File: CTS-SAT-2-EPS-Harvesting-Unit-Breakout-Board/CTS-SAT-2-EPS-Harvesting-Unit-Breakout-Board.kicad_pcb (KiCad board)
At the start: 2 copper layers, 60.2 x 19 mm, 9 parts, among them J1 Conn_01x02_Pin, U1 MAX9922EUB+T

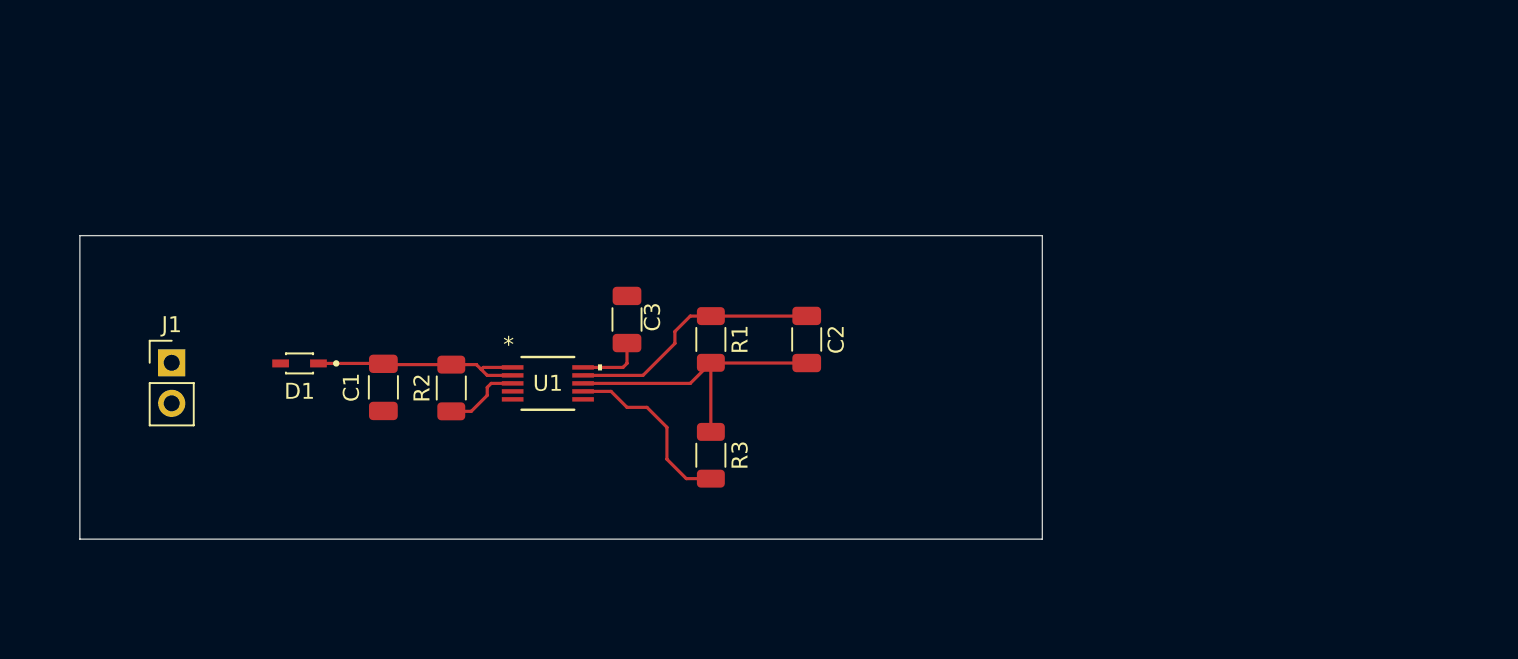
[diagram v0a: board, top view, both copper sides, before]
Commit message: update
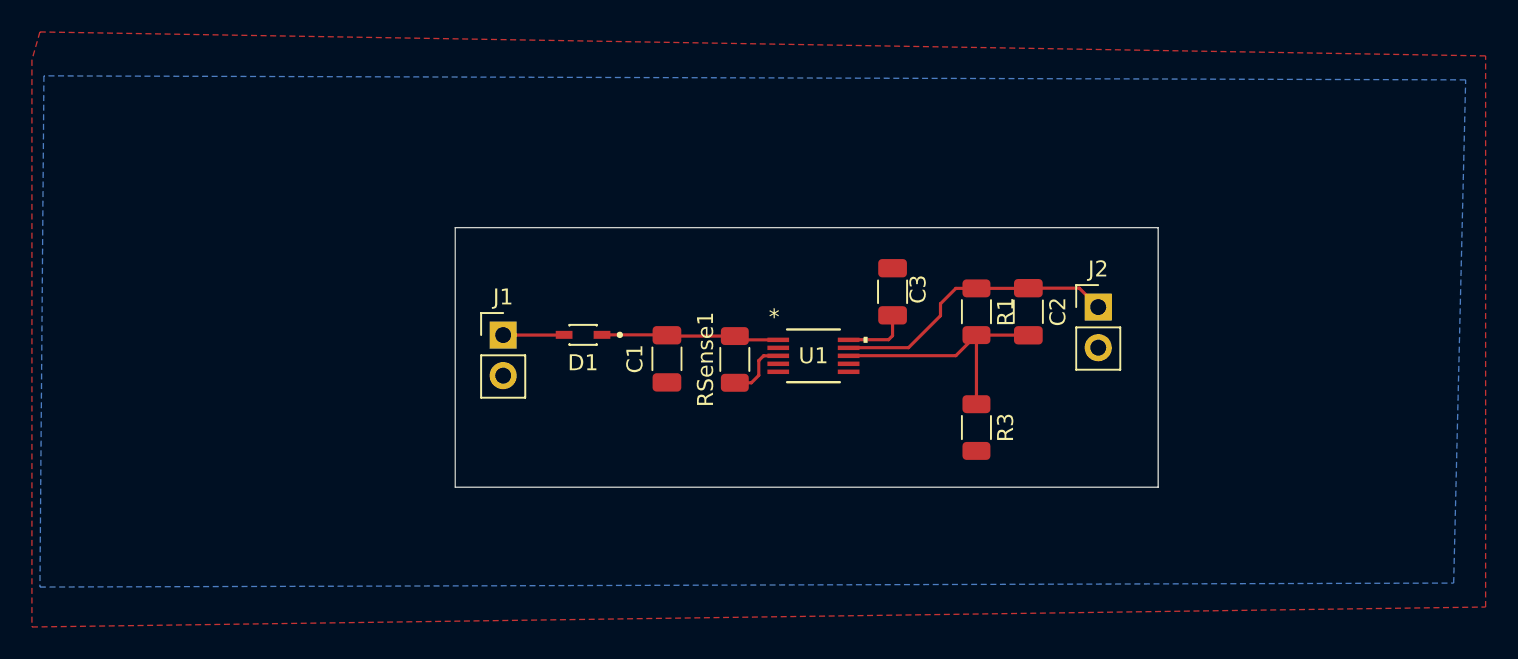
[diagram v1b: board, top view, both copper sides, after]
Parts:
- added J2: Conn_01x02_Pin, Connector_PinHeader_2.54mm:PinHeader_1x02_P2.54mm_Vertical, F.Cu at (167.2, 84.0)
- R1: value R -> 24k
- R3: value R -> 1k
- RSense1: renamed from R2; value 0.02 -> 1m
- moved J1 20.8 mm to (130.0, 85.7)
- moved C1 17.8 mm to (140.2, 87.2)
- moved D1 17.8 mm to (135.0, 85.7)
- moved RSense1 17.8 mm to (144.5, 87.2)
- moved C3 16.7 mm to (154.4, 83.0)
- moved R1 16.7 mm to (159.6, 84.3)
- moved R3 16.7 mm to (159.6, 91.5)
- moved U1 16.7 mm to (149.4, 87.0)
- moved C2 14.0 mm to (162.9, 84.3)
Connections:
- D1 pad A: unconnected-(D1-PadA) -> Net-(J1-Pin_1)
- J1 pad 1: unconnected-(J1-Pin_1-Pad1) -> Net-(J1-Pin_1)
- J1 pad 2: unconnected-(J1-Pin_2-Pad2) -> GNDA
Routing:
- net GNDA: track 11.4 -> 0.00 mm
- net Net-(J1-Pin_1): track 0.00 -> 3.82 mm
- net Net-(U1-RS+): track 14.6 -> 11.2 mm
- net Net-(U1-FB): track 18.9 -> 16.2 mm
- net Net-(J2-Pin_1): track 16.0 -> 18.1 mm
- net Net-(U1-RS-): track 4.86 -> 3.96 mm
- added copper zone on F.Cu, net +3.3V
- added copper zone on B.Cu, net GNDA
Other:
- board size 60.2 x 19 mm -> 44 x 16.2 mm
